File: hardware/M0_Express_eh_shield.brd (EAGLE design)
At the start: 51.3 x 53.3 mm, 30 parts, among them U1 TLV3691, U2 AB0815, U3 Value, U4 MIC841, U5 TPS781, X2 ABS05-32.768KHZ-9-T

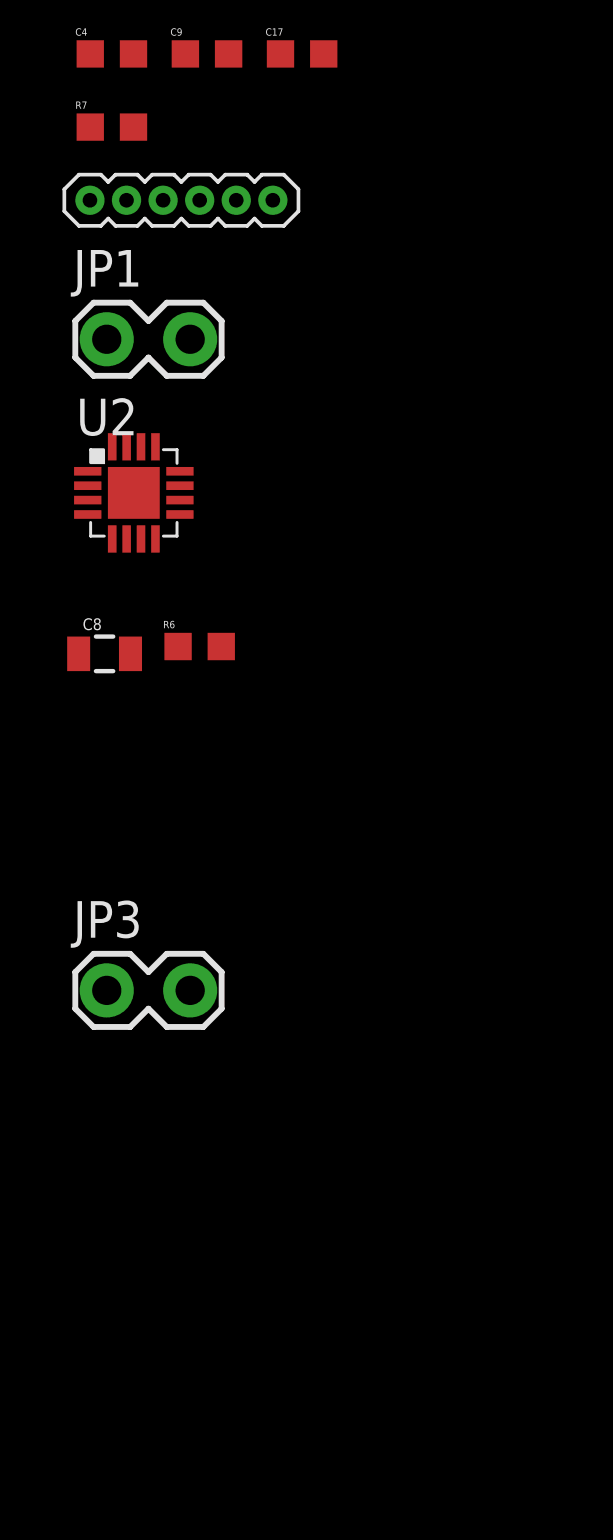
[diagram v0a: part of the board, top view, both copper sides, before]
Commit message: updates and programmer
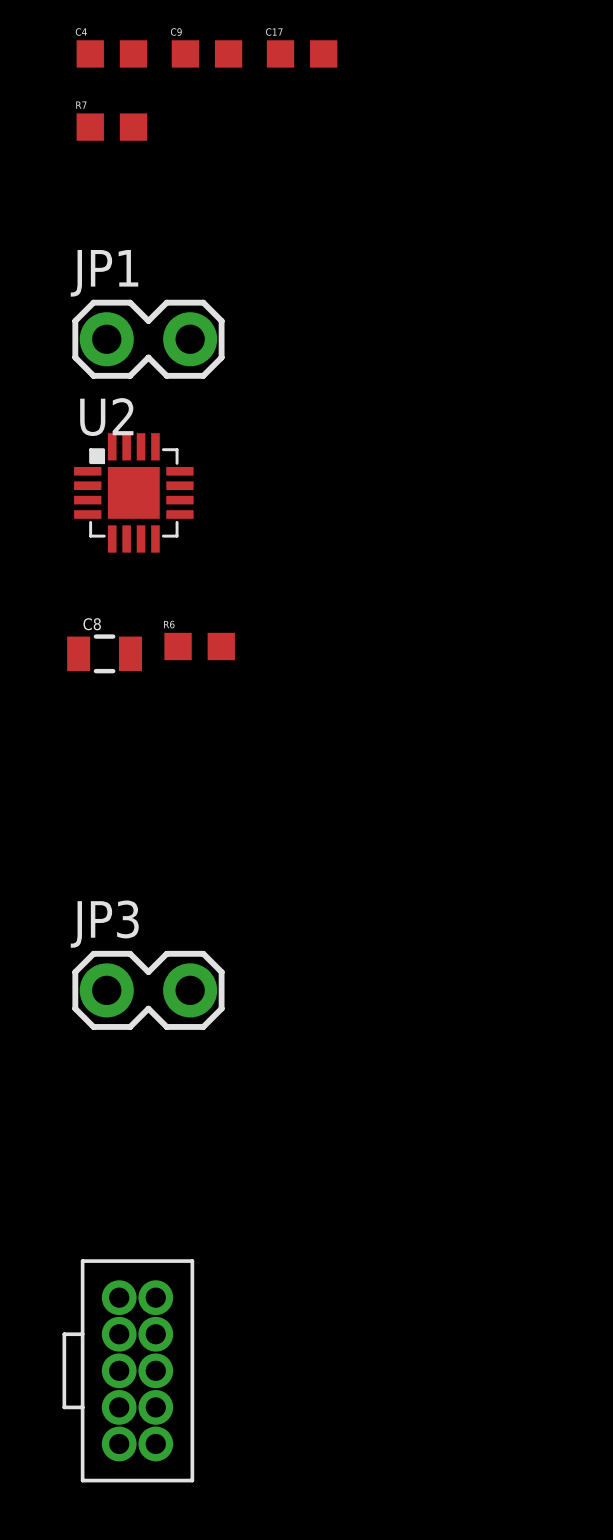
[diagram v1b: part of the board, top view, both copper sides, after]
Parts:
- removed JP11: (no value), SparkFun-Connectors:1X06-1.27MM
- added JP2: (no value), SparkFun-Connectors:2X5_1.27MM
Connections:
- net GND: now also JP2.10, JP2.9; no longer JP11.1
- net MSP430_RST: now also JP2.5, JP2.6; no longer JP11.3
- net MSP430_TEST: now also JP2.3, JP2.4; no longer JP11.2
- net RX_DEBUG: now also JP2.2; no longer JP11.4
- net TX_DEBUG: now also JP2.7, JP2.8; no longer JP11.5
- net VCC: now also JP2.1; no longer JP11.6
